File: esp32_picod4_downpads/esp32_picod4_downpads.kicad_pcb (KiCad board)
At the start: 2 copper layers, 72 x 62 mm, 84 parts, among them J1 PT0, J10 IO25, J11 IO26, J12 IO2, J13 MTDI, J14 EN, J15 IO0, J16 GND, J17 ‎2450AT42E0100E‎, J18 PGM_DBG, J19 Swadge_Parts_USB_B_Micro, J2 PT1, J3 PT2, J4 PT3, J5 PT4, J6 PT5, J7 PT6, J8 IO22, J9 IO23, K1 GND, K10 T6, K11 T7, K12 T8, K13 T9, K14 GND, K15 PT1, K16 PT2, K17 PT3, K18 PT4, K19 GND, K2 PT0, K20 3v3, K21 PT5, K22 G22, K23 G23, K24 G25, K25 G26, K26 PT6, K27 GND, K3 3v3, K4 ADC6, K5 ADC7, K6 GND, K7 T0, K8 T3, K9 T4, M1 GND, M2 GND, M3 GND, M4 GND, M5 GND, M6 GND, Q1 SS8050, Q2 SS8050, Q3 PMOS_GSD, Q4 PMOS_GSD, U1 ESP32-PICO-D4, U2 MCP1700-3302E_SOT23, U3 CP2104

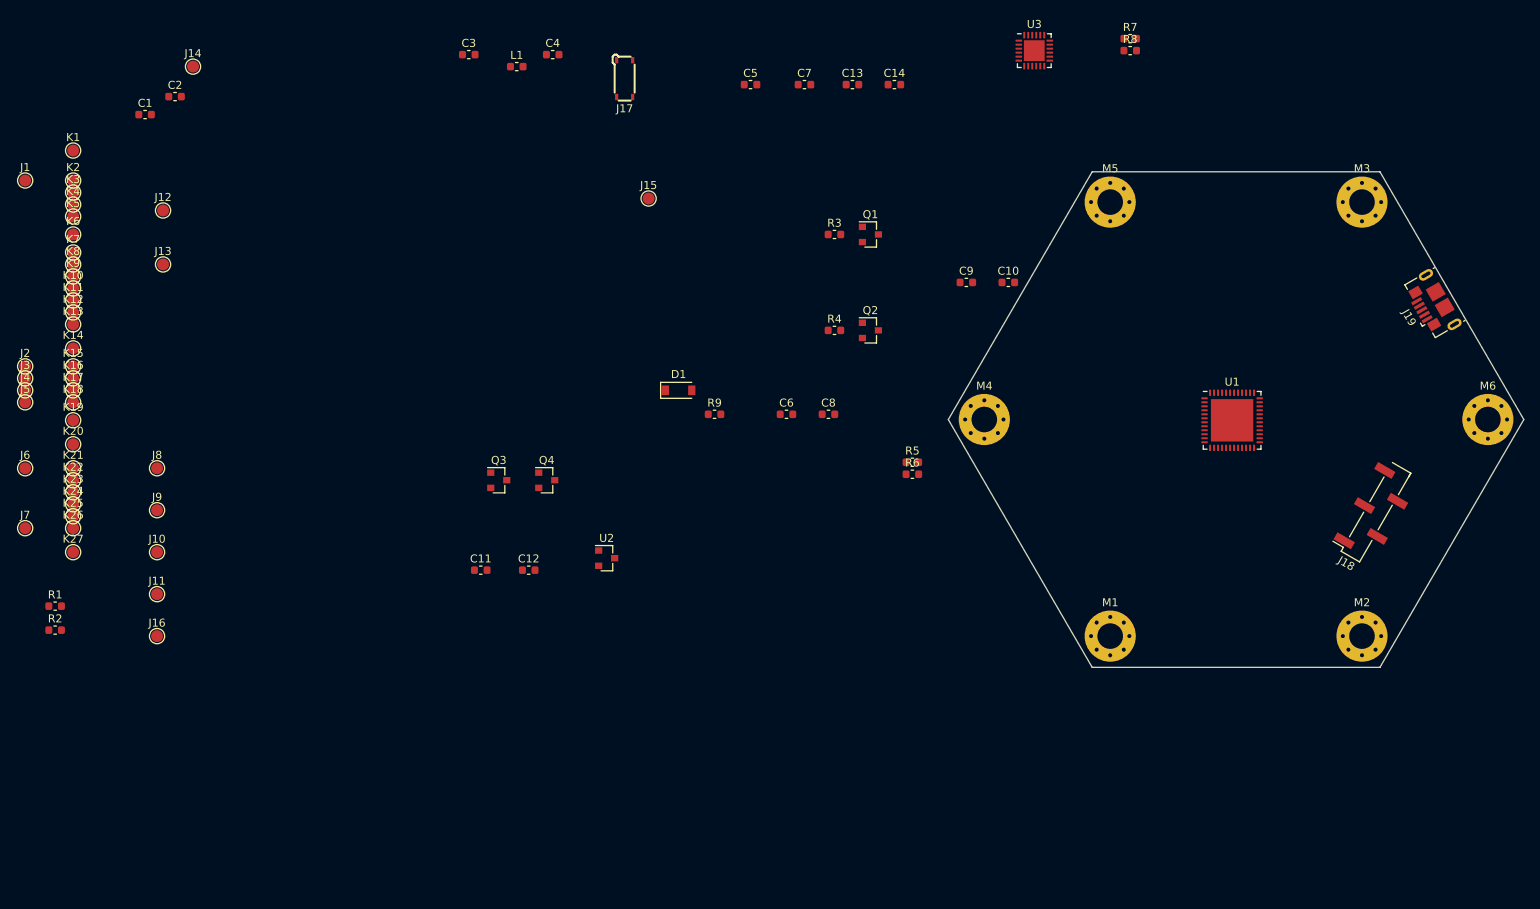
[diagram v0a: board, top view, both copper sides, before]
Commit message: Forgot to upload design
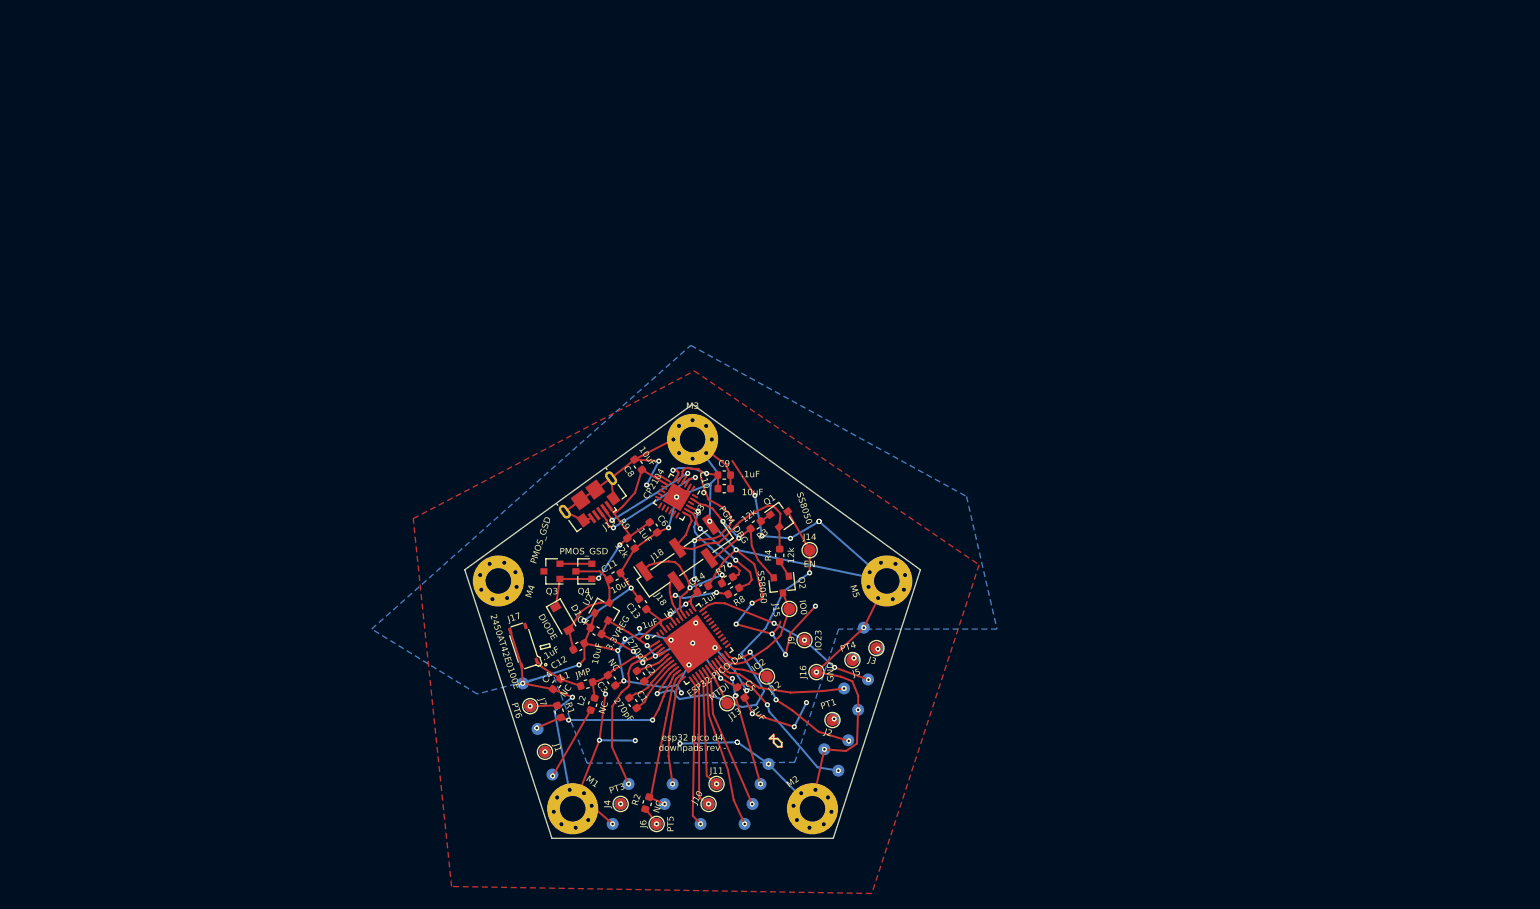
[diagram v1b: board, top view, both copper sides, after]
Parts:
- removed J8: IO22, TestPoint:TestPoint_Pad_D1.5mm
- removed M6: GND, MountingHole:MountingHole_3.2mm_M3_Pad_Via
- removed R5, R6: 0, Resistor_SMD:R_0603_1608Metric
- added K28: GND, TestPoint:TestPoint_Pad_D1.5mm, B.Cu at (78.8, 104.9)
- added L2: NC, Inductor_SMD:L_0603_1608Metric, F.Cu at (87.5, 107.5)
- K1, K10, K11, K12, K13, K14, K15, K16, K17, K18, K19, K2, K20, K21, K23, K24, K25, K26, K27, K3, K4, K5, K6, K7, K8, K9: moved to B.Cu
- K22: value G22 -> ANT; moved to B.Cu
- U2: value MCP1700-3302E_SOT23 -> 3.3VREG
- moved K7 114.6 mm to (119.5, 112.0), turned to 54 degrees
- moved J3 111.7 mm to (123.0, 100.5), turned to 162 degrees
- moved K6 110.5 mm to (121.4, 97.9), turned to 162 degrees
- moved J2 110.3 mm to (117.5, 109.5), turned to 162 degrees
- moved K8 110.1 mm to (119.0, 105.6), turned to 306 degrees
- moved J5 108.4 mm to (120.0, 102.0), turned to 198 degrees
- moved K1 108.0 mm to (90.0, 122.5), turned to 90 degrees
- moved J19 107.8 mm to (87.6, 82.3), turned to 216 degrees
- moved K9 106.9 mm to (108.5, 117.5), turned to 90 degrees
- moved K10 106.7 mm to (107.5, 120.0), turned to 90 degrees
- moved K14 106.5 mm to (116.5, 113.2), turned to 270 degrees
- moved K11 106.5 mm to (106.5, 122.5), turned to 90 degrees
- moved K16 106.2 mm to (123.2, 100.6), turned to 342 degrees
- moved K15 104.9 mm to (117.7, 109.4), turned to 126 degrees
- moved K19 104.7 mm to (120.7, 108.2), turned to 162 degrees
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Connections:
- K22 pad 1: GPIO22 -> Net-(K22-Pad1)
- U3 pad 3: Net-(R6-Pad2) -> Net-(J19-Pad3)
- U3 pad 4: Net-(R5-Pad1) -> Net-(J19-Pad2)
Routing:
- net GND: track 0.00 -> 357.0 mm, vias 0 -> 47
- net +3V3: track 0.00 -> 111.5 mm, vias 0 -> 12
- net #EN: track 0.00 -> 46.8 mm, vias 0 -> 2
- net VUSB: track 0.00 -> 34.8 mm, vias 0 -> 2
- net RTS: track 0.00 -> 24.6 mm
- net VSPIDGPIO23: track 0.00 -> 23.8 mm, vias 0 -> 4
- net ADC6: track 0.00 -> 21.9 mm, vias 0 -> 3
- net TOUCH0: track 0.00 -> 21.1 mm, vias 0 -> 3
- net DTR: track 0.00 -> 20.8 mm, vias 0 -> 2
- net TOUCH7: track 0.00 -> 20.0 mm, vias 0 -> 1
- net TOUCH8: track 0.00 -> 18.6 mm, vias 0 -> 1
- net TOUCH6: track 0.00 -> 18.1 mm, vias 0 -> 1
- net ADC7: track 0.00 -> 17.9 mm, vias 0 -> 1
- net U0RX: track 0.00 -> 17.4 mm, vias 0 -> 2
- net TOUCH3: track 0.00 -> 17.2 mm, vias 0 -> 1
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- added copper zone on B.Cu, net GND
- added copper zone on F.Cu, net GND
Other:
- board size 72 x 62 mm -> 57 x 54.3 mm
- net class Default: via_dia 0.8 -> 0.65; via_drill 0.4 -> 0.3
- board text added: "esp32 pico d4 downpads rev -"
